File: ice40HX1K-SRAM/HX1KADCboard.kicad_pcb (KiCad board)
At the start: 2 copper layers, 148 parts, among them J1 Conn_01x03_Male, J2 Conn_02x05_Odd_Even, J3 Conn_01x20_Male, J5 Conn_01x06_Male, J6 Conn_01x05, U1 LTC3406ES5, U10 FAN5341, U11 FAN5341, U12 FAN5341, U13 FAN5341, U2 MAX40200AUK, U3 LTC3406ES5, U4 MAX40200AUK, U5 AT25SF081-SSHD-X, U6 ICE40HX1K-VQ100(VQFP100), U7 AS7C34096A, U8 ATSAMD11D14A-SS, U9 BL652, X1 USBFCI_10103594_MILL, X2 ASE-10MHz, X3 ASE-10MHz, X4 ASE-10MHz, X5 ASV-xxxMHz, X6 ASV-xxxMHz, X7 ASV-xxxMHz

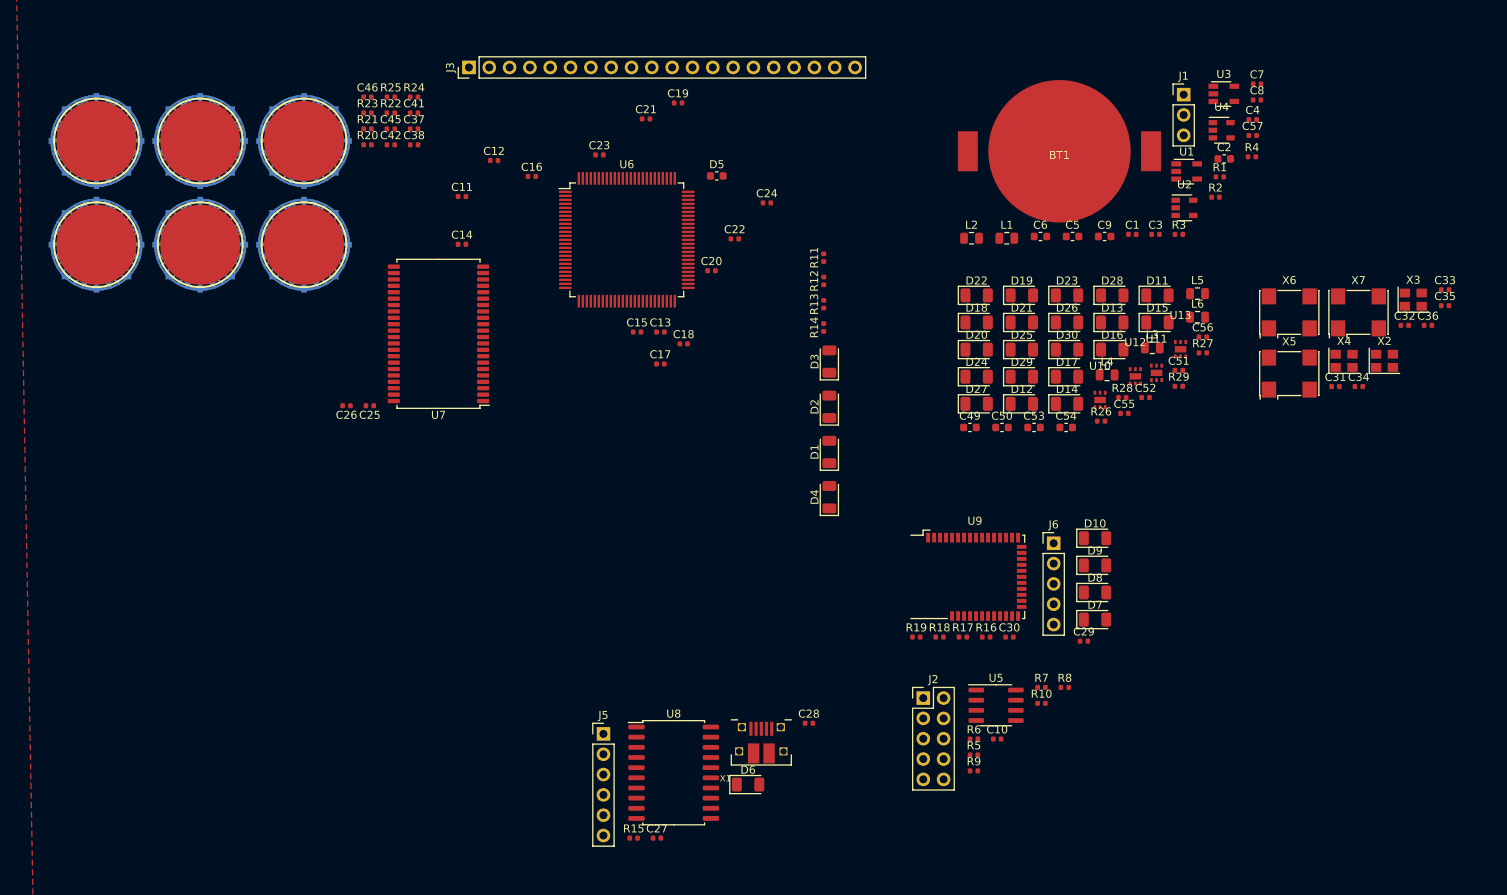
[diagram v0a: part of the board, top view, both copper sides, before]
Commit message: starting AutoRoute
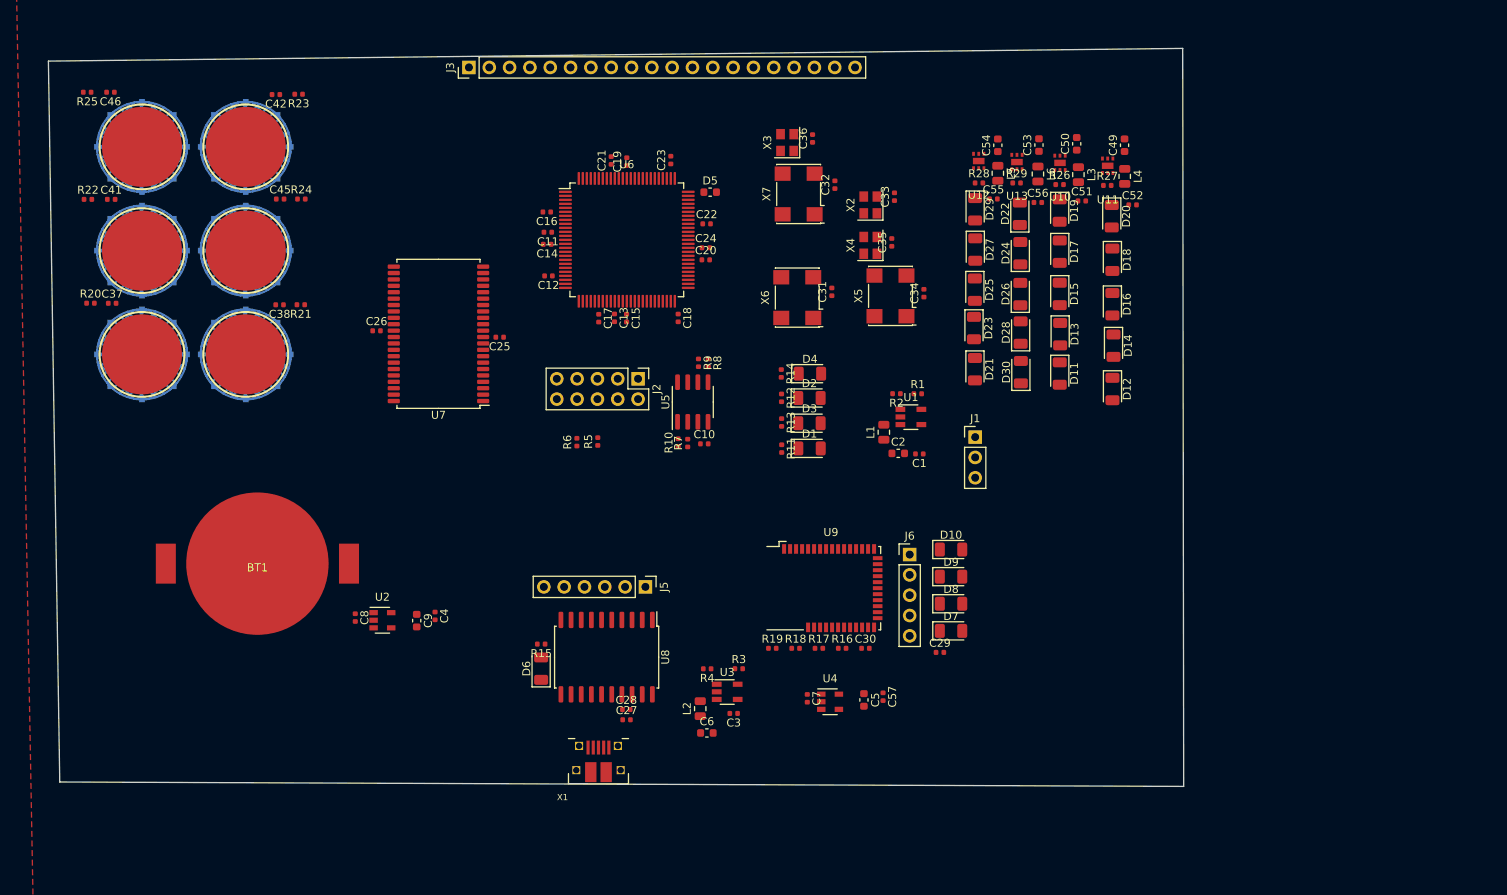
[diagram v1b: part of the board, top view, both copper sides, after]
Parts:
- moved C8 130.0 mm to (97.1, 111.4), turned to 270 degrees
- moved C4 119.6 mm to (107.1, 111.2), turned to 270 degrees
- moved BT1 112.7 mm to (84.9, 104.6)
- moved U2 112.7 mm to (100.5, 111.7)
- moved C9 98.5 mm to (104.8, 111.8), turned to 270 degrees
- moved U3 97.2 mm to (143.6, 120.7)
- moved C7 95.2 mm to (153.6, 121.5), turned to 270 degrees
- moved R4 93.4 mm to (141.1, 117.8), turned to 180 degrees
- moved U4 86.6 mm to (156.5, 121.9)
- moved C57 84.0 mm to (163.1, 121.3), turned to 270 degrees
- moved X3 80.7 mm to (151.1, 52.0), turned to 90 degrees
- moved C36 80.4 mm to (154.3, 51.5), turned to 90 degrees
- moved C3 79.8 mm to (144.4, 123.4), turned to 180 degrees
- moved R3 77.3 mm to (145.1, 117.8)
- moved C6 74.8 mm to (141.1, 125.8)
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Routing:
- added copper zone on In2.Cu, net +3V3
- added copper zone on In1.Cu, net GND
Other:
- board outline added: 141.9 x 92.2 mm
- copper layers 2 -> 4
